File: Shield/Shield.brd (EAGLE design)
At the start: 160 x 100 mm, 25 parts

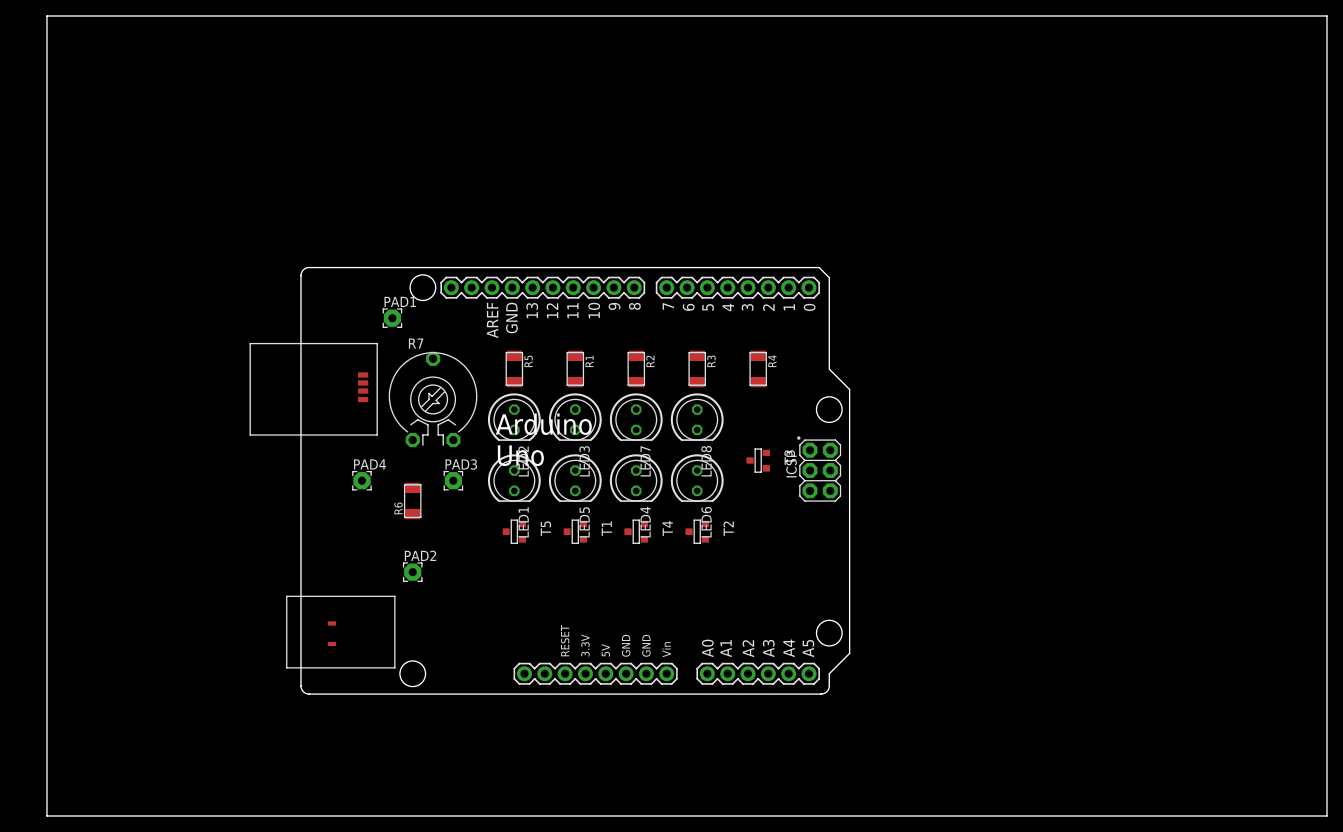
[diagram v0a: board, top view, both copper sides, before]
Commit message: Update Shield.brd
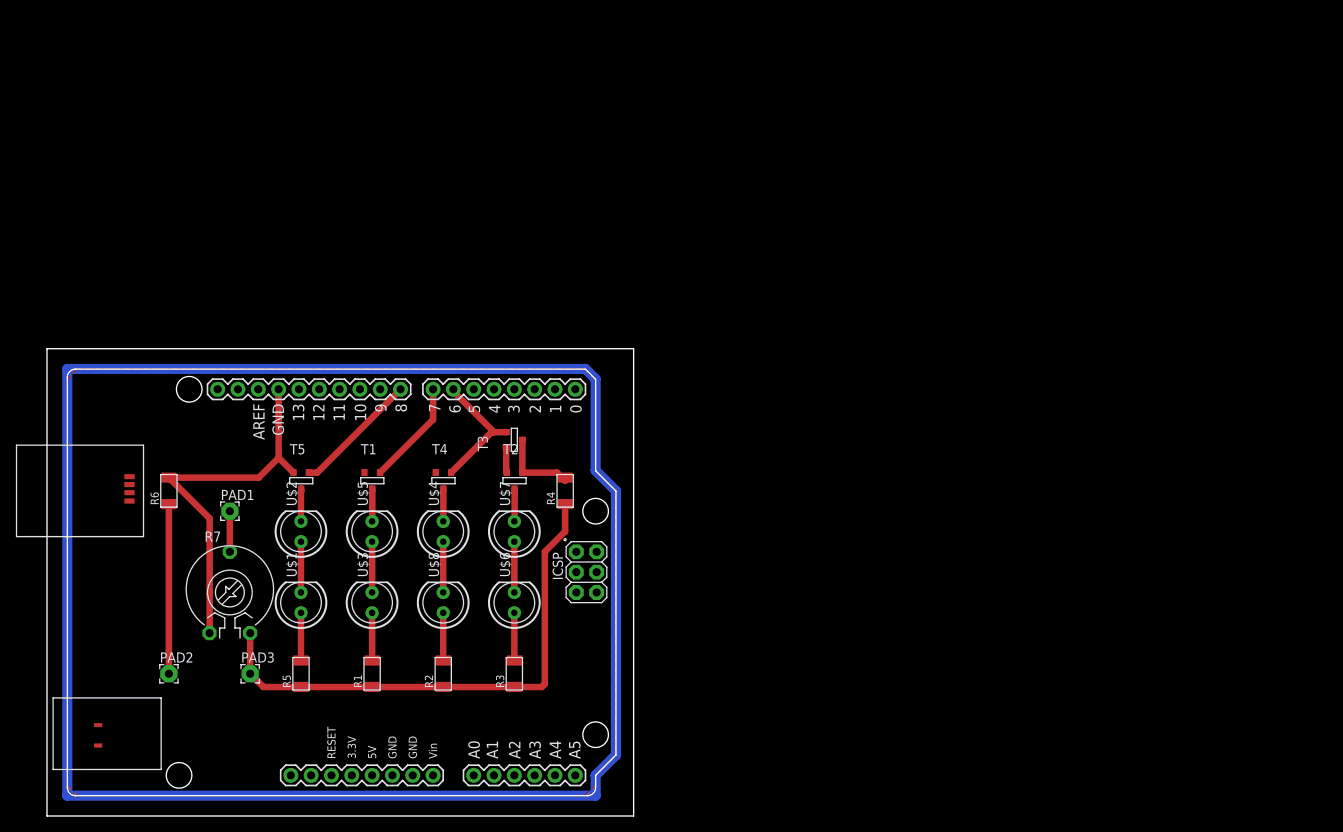
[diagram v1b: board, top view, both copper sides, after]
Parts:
- removed LED1, LED2, LED3, LED4, LED5, LED6, LED7, LED8: (no value), led:LED5MM
- removed PAD4: (no value), wirepad:2,15/1,0
- added U$1, U$2, U$3, U$4, U$5, U$6, U$7, U$8: LED5MM, fab:5MM
- moved R5 46.5 mm to (31.8, 17.8), turned to 90 degrees
- moved R1 45.8 mm to (40.6, 17.8), turned to 90 degrees
- moved R2 45.1 mm to (49.5, 17.8), turned to 90 degrees
- moved R3 44.4 mm to (58.4, 17.8), turned to 90 degrees
- moved R7 35.0 mm to (22.9, 27.9)
- moved PAD3 35.0 mm to (25.4, 17.8)
- moved PAD2 33.0 mm to (15.2, 17.8)
- moved PCB1 31.9 mm to (2.54, 2.54)
- moved PAD1 31.5 mm to (22.9, 38.1)
- moved T3 30.6 mm to (58.4, 47.0), turned to 90 degrees
- moved R6 30.5 mm to (15.2, 40.6)
- moved R4 28.5 mm to (64.8, 40.6), turned to 90 degrees
- moved T5 27.4 mm to (31.8, 41.9), turned to 0 degrees
- moved T1 26.2 mm to (40.6, 41.9), turned to 0 degrees
- moved T4 25.0 mm to (49.5, 41.9), turned to 0 degrees
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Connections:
- removed net N$16: PAD4.1, R6.2, R7.1, T1.2, T2.2, T3.2, T4.2, T5.2
- new net GND: PCB1.GND, PCB1.GND., PCB1.GND.., R6.2, R7.1, T1.2, T2.2, T3.2, T4.2, T5.2
- net N$1: now also U$1.OUT, U$2.IN; no longer LED1.A, LED2.K
- net N$10: now also U$2.OUT; no longer LED1.K
- net N$11: now also U$5.OUT; no longer LED5.K
- net N$12: now also U$4.OUT; no longer LED4.K
- net N$14: now also U$7.OUT; no longer LED6.K
- net N$2: now also U$3.OUT, U$5.IN; no longer LED3.K, LED5.A
- net N$3: now also U$4.IN, U$8.OUT; no longer LED4.A, LED7.K
- net N$4: now also U$6.OUT, U$7.IN; no longer LED6.A, LED8.K
- net N$5: now also U$1.IN; no longer LED2.A
- net N$6: now also U$3.IN; no longer LED3.A
- net N$7: now also U$8.IN; no longer LED7.A
- net N$8: now also U$6.IN; no longer LED8.A
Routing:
- net N$15: track 0.00 -> 240.1 mm
- net N$20: track 0.00 -> 66.3 mm
- net GND: track 0.00 -> 50.6 mm
- net N$13: track 0.00 -> 21.2 mm
- net N$19: track 0.00 -> 16.4 mm
- net N$17: track 0.00 -> 15.8 mm
- net N$18: track 0.00 -> 13.2 mm
- net N$21: track 0.00 -> 10.3 mm
- net N$4: track 0.00 -> 6.35 mm
- net N$3: track 0.00 -> 6.35 mm
- net N$2: track 0.00 -> 6.35 mm
- net N$1: track 0.00 -> 6.35 mm
- net N$8: track 0.00 -> 5.97 mm
- net N$7: track 0.00 -> 5.97 mm
- net N$6: track 0.00 -> 5.97 mm
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- added copper zone on layer 1, net GND
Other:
- board size 160 x 100 mm -> 73.3 x 58.4 mm
